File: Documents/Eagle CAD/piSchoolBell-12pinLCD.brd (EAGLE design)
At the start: 65 x 56 mm, 17 parts, among them J1 455-1750-1-ND, X1 RASPI_BOARD_B+#_H

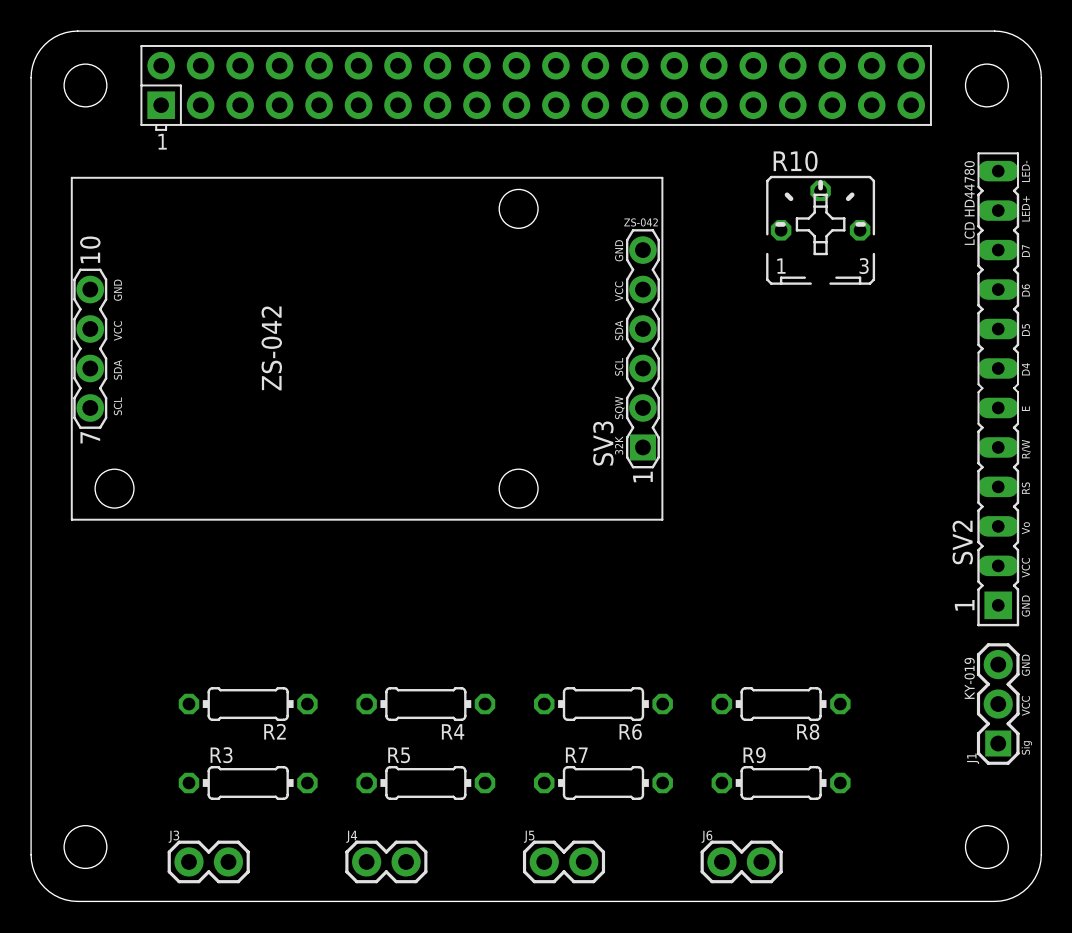
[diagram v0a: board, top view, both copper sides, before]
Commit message: Routed PCB
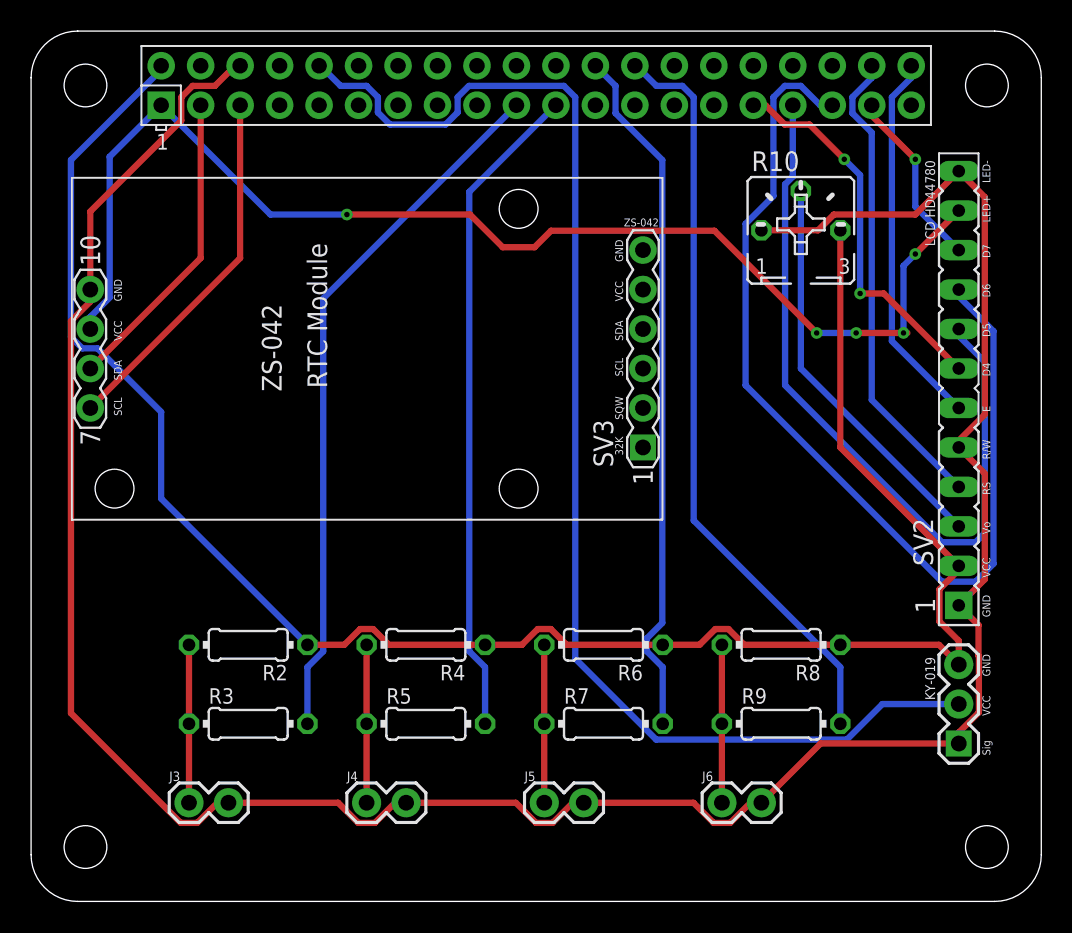
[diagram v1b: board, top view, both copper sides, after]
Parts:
- moved R2 3.81 mm to (-64.8, 17.8)
- moved R4 3.81 mm to (-53.3, 17.8)
- moved R6 3.81 mm to (-41.9, 17.8)
- moved R8 3.81 mm to (-30.5, 17.8)
- moved J3 3.81 mm to (-68.6, 7.62)
- moved J4 3.81 mm to (-57.1, 7.62)
- moved J5 3.81 mm to (-45.7, 7.62)
- moved J6 3.81 mm to (-34.3, 7.62)
- moved R3 3.81 mm to (-64.8, 12.7)
- moved R5 3.81 mm to (-53.3, 12.7)
- moved R7 3.81 mm to (-41.9, 12.7)
- moved R9 3.81 mm to (-30.5, 12.7)
- moved J1 2.54 mm to (-19.1, 11.4)
- moved SV2 2.54 mm to (-19.1, 20.3)
- moved R10 1.27 mm to (-29.2, 44.5)
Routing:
- net N$27: track 0.00 -> 166.6 mm
- net N$15: track 0.00 -> 123.6 mm
- net N$28: track 0.00 -> 84.4 mm
- net N$18: track 0.00 -> 80.6 mm, vias 0 -> 5
- net N$14: track 0.00 -> 64.1 mm
- net N$13: track 0.00 -> 49.3 mm
- net N$25: track 0.00 -> 48.1 mm
- net N$7: track 0.00 -> 45.4 mm
- net N$24: track 0.00 -> 45.0 mm
- net N$23: track 0.00 -> 42.5 mm
- net N$9: track 0.00 -> 30.5 mm
- net N$1: track 0.00 -> 25.8 mm
- net N$12: track 0.00 -> 24.7 mm, vias 0 -> 2
- net N$11: track 0.00 -> 24.3 mm
- net N$4: track 0.00 -> 23.5 mm
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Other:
- board text added: "Design: Jon Sagebrand jonsagebrand@gmail.com piSchoolBell @ https://github.com/jonsag/piSchoolBell"
